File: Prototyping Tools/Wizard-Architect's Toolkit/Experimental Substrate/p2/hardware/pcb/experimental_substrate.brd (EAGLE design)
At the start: 19.7 x 108 mm, 28 parts, among them J1 EURO_POWER

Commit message: Add logo
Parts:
- added U$26: (no value), SonicAthame:LOGO-30MIL-BSILK
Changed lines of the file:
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@@
 </layers>
 <board>
-<fusionsync huburn="a.cGVyc29uYWw6dWUyZGY0M2Ex" projecturn="a.cGVyc29uYWw6dWUyZGY0M2ExIzIwMjAwODA5MzIyMjM2MzA2" f3durn="urn:adsk.wipprod:dm.lineage:Q2m1L6VbTlGJL3gwAvu5pw" pcbguid="ba5cba06-7faf-45c1-a827-196ae48076d6" lastpulledtime="" lastsyncedchangeguid="a4e57447-2fd9-805a-3b14-6fc53e18663e"/>
+<fusionsync huburn="a.cGVyc29uYWw6dWUyZGY0M2Ex" projecturn="a.cGVyc29uYWw6dWUyZGY0M2ExIzIwMjAwODA5MzIyMjM2MzA2" f3durn="urn:adsk.wipprod:dm.lineage:Q2m1L6VbTlGJL3gwAvu5pw" pcbguid="ba5cba06-7faf-45c1-a827-196ae48076d6" lastpulledtime="" lastsyncedchangeguid="2ea98b64-b3de-7964-73d5-6c74d01ecbd5"/>
 <plain>
 <wire x1="19.685" y1="118.11" x2="0.635" y2="118.11" width="0" layer="20"/>
@@
 <text x="1.905" y="109.22" size="0.6096" layer="25" align="top-center">10uF</text>
 <text x="17.145" y="109.22" size="0.6096" layer="25" align="top-center">10uF</text>
-<text x="9.525" y="109.22" size="1.016" layer="26" rot="MR0" align="center">Wizard-Architect's Toolkit
+<text x="9.525" y="109.22" size="0.6096" layer="26" rot="MR0" align="center">Wizard-Architect's Toolkit
 Experimental Substrate</text>
 <text x="9.525" y="109.22" size="0.4064" layer="26" rot="MR180" align="center">Prototype v2</text>
@@
 </element>
 <element name="J1" library="SonicAthame" library_urn="urn:adsk.eagle:library:22327399" package="EURO_POWER" package3d_urn="urn:adsk.eagle:package:26183621/4" value="EURO_POWER" x="9.525" y="114.935" smashed="yes" rot="MR0">
-<attribute name="NAME" x="2.421" y="114.935" size="1.27" layer="28" rot="MR270" align="bottom-center"/>
+<attribute name="NAME" x="2.929" y="116.967" size="1.27" layer="28" rot="MR270" align="bottom-center"/>
 </element>
 <element name="U$1" library="SonicAthame" library_urn="urn:adsk.eagle:library:22327399" package="PANEL_REF_4U" package3d_urn="urn:adsk.eagle:package:26352493/3" value="" x="0" y="0" smashed="yes"/>
@@
 <element name="U$24" library="SonicAthame" library_urn="urn:adsk.eagle:library:22327399" package="LOGO-65MIL-TSILK" package3d_urn="urn:adsk.eagle:package:26328147/3" value="" x="13.335" y="10.795" smashed="yes" rot="R45"/>
 <element name="U$25" library="SonicAthame" library_urn="urn:adsk.eagle:library:22327399" package="LOGO-65MIL-TSILK" package3d_urn="urn:adsk.eagle:package:26328147/3" value="" x="3.81" y="10.795" smashed="yes" rot="R45"/>
+<element name="U$26" library="SonicAthame" library_urn="urn:adsk.eagle:library:22327399" package="LOGO-30MIL-BSILK" package3d_urn="urn:adsk.eagle:package:26382639/1" value="" x="18.288" y="109.601" smashed="yes" rot="R270"/>
 </elements>
 <signals>

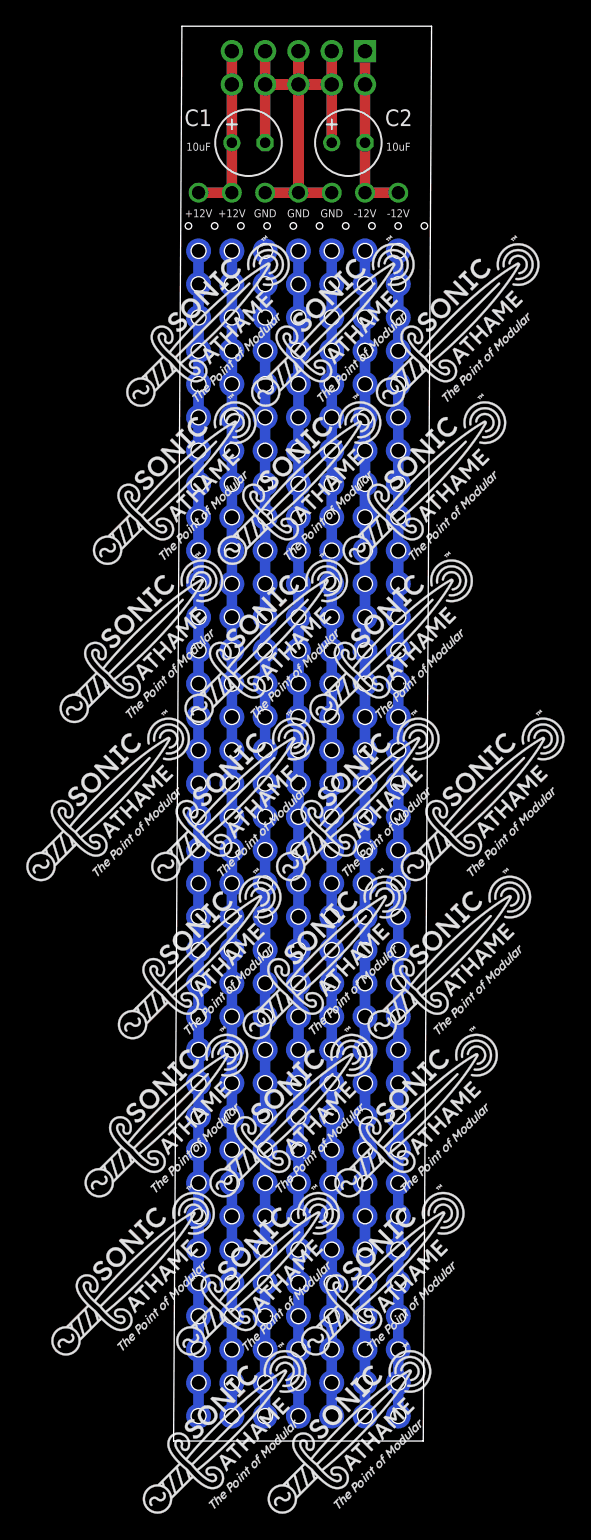
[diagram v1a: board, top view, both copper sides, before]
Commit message: Extreme improvements on stripboard v2
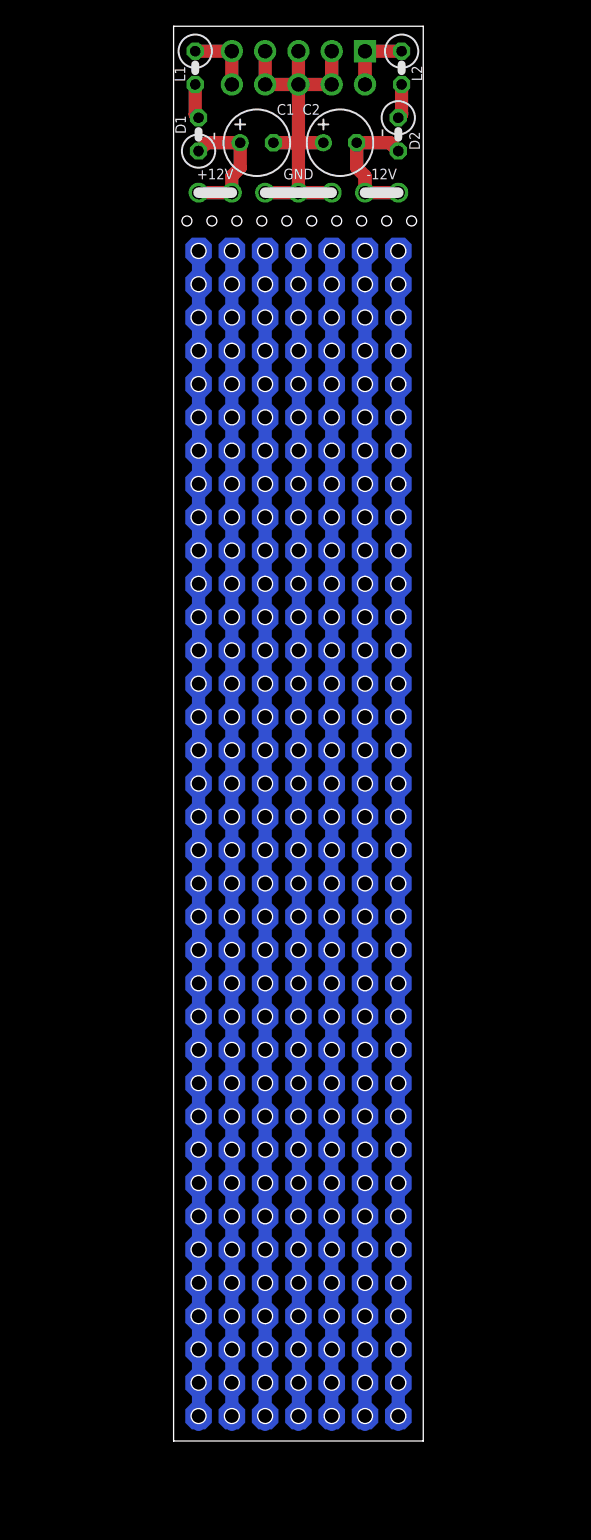
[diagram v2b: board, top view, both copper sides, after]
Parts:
- added D1, D2: SCHOTTKY_THT, SonicAthame:0207/2V-POL
- added L1, L2: FERRITE_THT, SonicAthame:0207/2V
- added U$100, U$101, U$102, U$103, U$104, U$105, U$106, U$107, U$108, U$109, U$110, U$111, U$112, U$113, U$114, U$115, U$116, U$117, U$118, U$119, U$120, U$121, U$122, U$123, U$124, U$125, U$126, U$127, U$128, U$129, U$130, U$131, U$132, U$133, U$134, U$135, U$136, U$137, U$138, U$139, U$140, U$141, U$142, U$143, U$144, U$145, U$146, U$147, U$148, U$149, U$150, U$151, U$152, U$153, U$154, U$155, U$156, U$157, U$158, U$159, U$160, U$161, U$162, U$163, U$164, U$165, U$166, U$167, U$168, U$169, U$170, U$171, U$172, U$173, U$174, U$175, U$176, U$177, U$178, U$179, U$180, U$181, U$182, U$183, U$184, U$185, U$186, U$187, U$188, U$189, U$190, U$191, U$192, U$193, U$194, U$195, U$196, U$197, U$198, U$199, U$200, U$201, U$202, U$203, U$204, U$205, U$206, U$207, U$208, U$209, U$210, U$211, U$212, U$213, U$214, U$215, U$216, U$217, U$218, U$219, U$220, U$221, U$222, U$223, U$224, U$225, U$226, U$227, U$228, U$229, U$230, U$231, U$232, U$233, U$234, U$235, U$236, U$237, U$238, U$239, U$240, U$241, U$242, U$243, U$244, U$245, U$246, U$247, U$248, U$249, U$250, U$251, U$252, U$253, U$27, U$28, U$29, U$30, U$31, U$32, U$33, U$34, U$35, U$36, U$37, U$38, U$39, U$40, U$41, U$42, U$43, U$44, U$45, U$46, U$47, U$48, U$49, U$50, U$51, U$52, U$53, U$54, U$55, U$56, U$57, U$58, U$59, U$60, U$61, U$62, U$63, U$64, U$65, U$66, U$67, U$68, U$69, U$70, U$71, U$72, U$73, U$74, U$75, U$76, U$77, U$78, U$79, U$80, U$81, U$82, U$83, U$84, U$85, U$86, U$87, U$88, U$89, U$90, U$91, U$92, U$93, U$94, U$95, U$96, U$97, U$98, U$99: (no value), SonicAthame:PAD_THT_0.1IN_NONPLATED
- U$10, U$11, U$12, U$13, U$14, U$15, U$16, U$17, U$18, U$19, U$2, U$20, U$21, U$22, U$23, U$24, U$25, U$3, U$4, U$5, U$6, U$7, U$8, U$9: device SonicAthame:LOGO-65MIL-TSILK -> SonicAthame:PAD_THT_0.1IN_NONPLATED
- U$26: device SonicAthame:LOGO-30MIL-BSILK -> SonicAthame:PAD_THT_0.1IN_NONPLATED
- moved U$25 83.0 mm to (12.1, 93.3), flipped to the bottom, turned to 0 degrees
- moved U$24 82.6 mm to (14.6, 93.3), flipped to the bottom, turned to 0 degrees
- moved U$22 75.8 mm to (17.1, 95.9), flipped to the bottom, turned to 0 degrees
- moved U$21 73.5 mm to (14.6, 95.9), flipped to the bottom, turned to 0 degrees
- moved U$23 70.5 mm to (17.1, 93.3), flipped to the bottom, turned to 0 degrees
- moved U$19 61.8 mm to (9.53, 95.9), flipped to the bottom, turned to 0 degrees
- moved U$20 61.3 mm to (12.1, 95.9), flipped to the bottom, turned to 0 degrees
- moved U$18 61.0 mm to (6.99, 95.9), flipped to the bottom, turned to 0 degrees
- moved U$15 52.3 mm to (1.91, 98.4), flipped to the bottom, turned to 0 degrees
- moved U$17 51.6 mm to (4.45, 95.9), flipped to the bottom, turned to 0 degrees
- moved U$16 48.9 mm to (1.91, 95.9), flipped to the bottom, turned to 0 degrees
- moved U$14 43.7 mm to (4.45, 98.4), flipped to the bottom, turned to 0 degrees
- moved U$12 42.0 mm to (9.53, 98.4), flipped to the bottom, turned to 0 degrees
- moved U$11 40.1 mm to (12.1, 98.4), flipped to the bottom, turned to 0 degrees
- moved U$13 40.0 mm to (6.99, 98.4), flipped to the bottom, turned to 0 degrees
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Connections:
- new net N$10: J1.1, J1.10, L2.1
- new net N$11: J1.5, J1.6, L1.1
- new net N$8: D1.A, L1.2
- new net N$9: D2.C, L2.2
- net +12V: now also D1.C; no longer J1.5, J1.6
- net -12V: now also D2.A; no longer J1.1, J1.10
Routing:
- net N$11: track 0.00 -> 5.33 mm
- net N$10: track 0.00 -> 5.33 mm
- net GND: track 34.9 -> 29.8 mm
- net -12V: track 13.3 -> 10.1 mm
- net +12V: track 13.3 -> 10.1 mm
- net N$9: track 0.00 -> 2.65 mm
- net N$8: track 0.00 -> 2.65 mm
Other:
- board size 19.7 x 108 mm -> 19.1 x 108 mm
- board text added: "STRIPE"
- board text removed: "10uF"
